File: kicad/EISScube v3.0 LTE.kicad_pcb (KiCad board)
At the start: 4 copper layers, 100 x 72 mm, 255 parts, among them J1 Boot, J2 UART, J3 JTag, J4 SIM_Card_w_det_sw, J5 USB_B_Mini, J6 Screw_Terminal_01x08, K1 SANYOU_SRD_Form_C, Q2 GSM3612PJZF, Q3 GSM3612PJZF, Q4 GSM3612PJZF, Q5 GSM3612PJZF, SW1 Reset, U1 STM32L051C8Tx, U2 SN74LV1T34DBVR, U3 U-Blox-SARA-R4, U4 LM2576HVS-12, U5 MIC29302WU-TR, U6 L7805, U7 LM1117-3.3, U8 LM1117-1.8, U9 LTV-357T, Y1 12MHz, Y2 32.768KHz

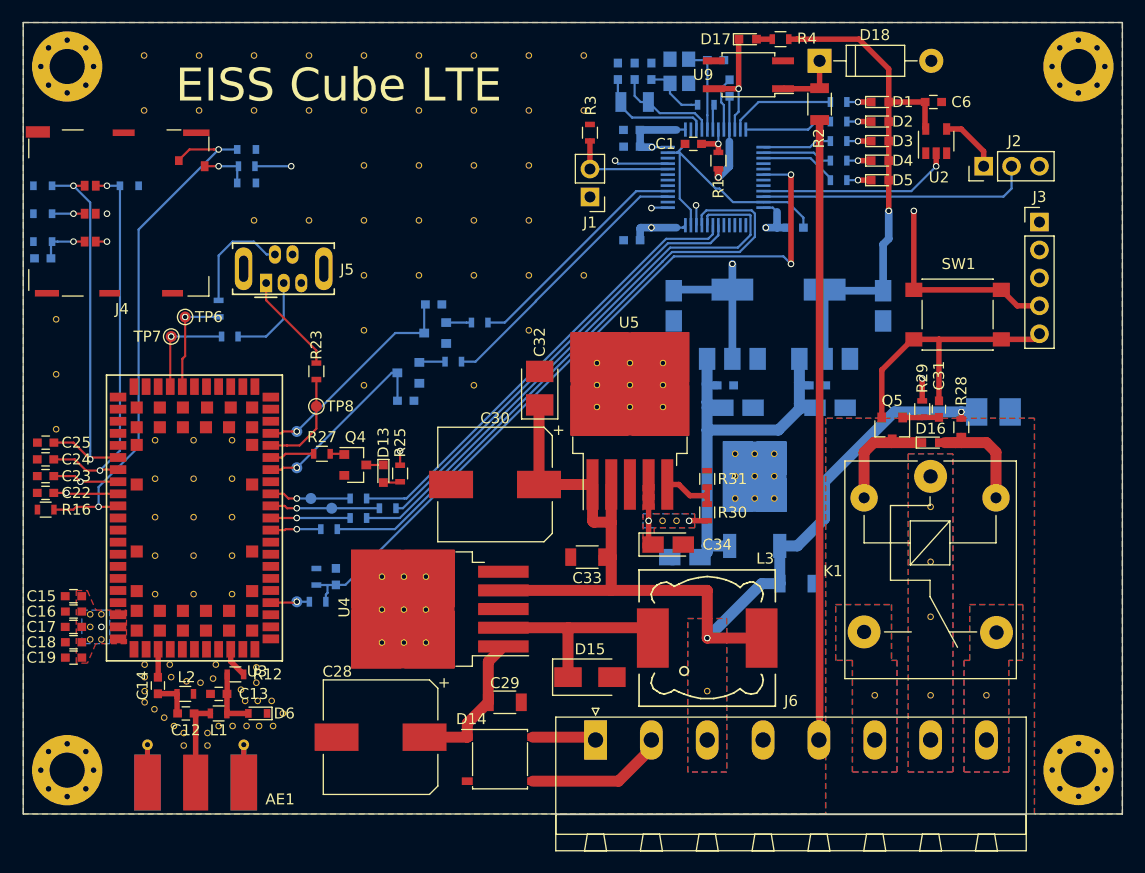
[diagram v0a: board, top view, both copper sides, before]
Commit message: Changes for enclosure case
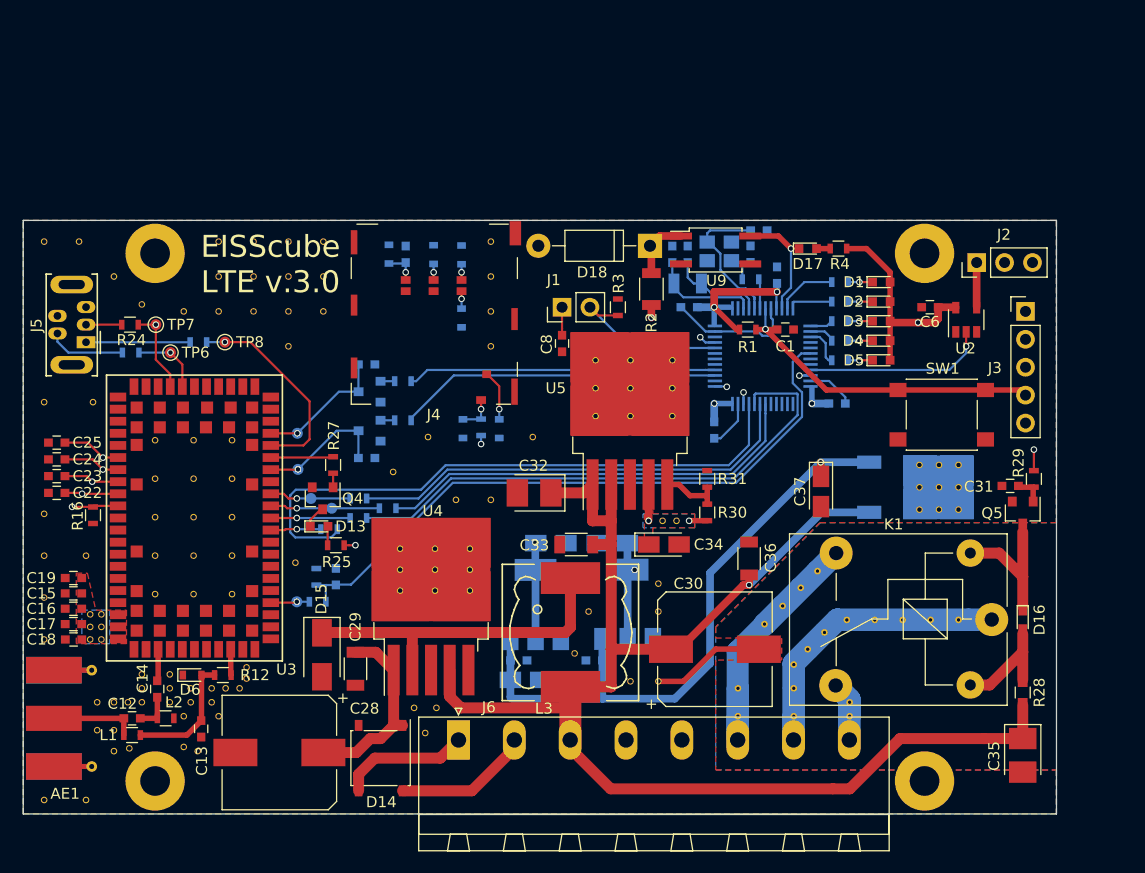
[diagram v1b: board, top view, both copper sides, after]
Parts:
- removed the REF** at (160.0, 122.2)
- removed the REF** at (180.3, 122.6)
- removed the REF** at (180.3, 115.4)
- removed the REF** at (180.3, 110.4)
- removed the REF** at (180.3, 105.4)
- removed the REF** at (185.4, 122.6)
- removed the REF** at (175.3, 122.6)
- removed the REF** at (128.8, 94.3)
- removed the REF** at (138.8, 94.3)
- removed the REF** at (143.8, 89.3)
- removed the REF** at (120.4, 123.1)
- removed the REF** at (121.4, 124.2)
- removed the REF** at (114.6, 126.0)
- removed the REF** at (115.1, 121.0)
- added REF**: VIA-0.6mm, EISScube_LTE:VIA-0.6mm, F.Cu at (134.4, 126.0)
- added REF**: VIA-0.6mm, EISScube_LTE:VIA-0.6mm, F.Cu at (104.9, 116.3)
- added REF**: VIA-0.6mm, EISScube_LTE:VIA-0.6mm, F.Cu at (170.1, 111.3)
- added REF**: VIA-0.6mm, EISScube_LTE:VIA-0.6mm, F.Cu at (168.5, 112.8)
- added REF**: VIA-0.6mm, EISScube_LTE:VIA-0.6mm, F.Cu at (166.9, 114.4)
- added REF**: VIA-0.6mm, EISScube_LTE:VIA-0.6mm, F.Cu at (165.2, 116.1)
- added REF**: VIA-0.6mm, EISScube_LTE:VIA-0.6mm, F.Cu at (173.0, 124.5)
- added REF**: VIA-0.6mm, EISScube_LTE:VIA-0.6mm, F.Cu at (173.0, 123.2)
- added REF**: VIA-0.6mm, EISScube_LTE:VIA-0.6mm, F.Cu at (162.8, 121.9)
- added REF**: VIA-0.6mm, EISScube_LTE:VIA-0.6mm, F.Cu at (162.8, 124.5)
- added REF**: VIA-0.6mm, EISScube_LTE:VIA-0.6mm, F.Cu at (169.2, 118.4)
- added REF**: VIA-0.6mm, EISScube_LTE:VIA-0.6mm, F.Cu at (167.9, 124.5)
- added REF**: VIA-0.6mm, EISScube_LTE:VIA-0.6mm, F.Cu at (175.3, 115.7)
- added REF**: VIA-0.6mm, EISScube_LTE:VIA-0.6mm, F.Cu at (135.4, 123.7)
- added REF**: VIA-0.6mm, EISScube_LTE:VIA-0.6mm, F.Cu at (177.8, 115.7)
- added REF**: VIA-0.6mm, EISScube_LTE:VIA-0.6mm, F.Cu at (167.9, 121.9)
- added REF**: VIA-0.6mm, EISScube_LTE:VIA-0.6mm, F.Cu at (167.9, 119.8)
- added REF**: VIA-0.6mm, EISScube_LTE:VIA-0.6mm, F.Cu at (170.7, 116.8)
- added REF**: VIA-0.6mm, EISScube_LTE:VIA-0.6mm, F.Cu at (172.7, 115.7)
- added REF**: VIA-0.6mm, EISScube_LTE:VIA-0.6mm, F.Cu at (180.3, 115.7)
- added REF**: VIA-0.6mm, EISScube_LTE:VIA-0.6mm, F.Cu at (182.9, 115.7)
- added REF**: VIA-0.6mm, EISScube_LTE:VIA-0.6mm, F.Cu at (133.3, 123.7)
- added REF**: VIA-0.6mm, EISScube_LTE:VIA-0.6mm, F.Cu at (148.0, 118.7)
- added REF**: VIA-0.6mm, EISScube_LTE:VIA-0.6mm, F.Cu at (149.2, 114.9)
- added REF**: VIA-0.6mm, EISScube_LTE:VIA-0.6mm, F.Cu at (155.6, 112.4)
- added REF**: VIA-0.6mm, EISScube_LTE:VIA-0.6mm, F.Cu at (155.6, 114.9)
- added REF**: VIA-0.6mm, EISScube_LTE:VIA-0.6mm, F.Cu at (155.6, 121.3)
- added REF**: VIA-0.6mm, EISScube_LTE:VIA-0.6mm, F.Cu at (153.0, 121.3)
- AE1: value Antenna_Shield -> Antenna
- C35, C36, C37, C8, R24: moved to F.Cu
- J4: value SIM_Card_w_det_sw -> SIM card holder
- J6: value Screw_Terminal_01x08 -> Connector 1 x 8
- K1: value SANYOU_SRD_Form_C -> SRD Form C
- R23: moved to B.Cu
- REF**: footprint Mounting_Holes:MountingHole_3.2mm_M3_Pad_Via -> Mounting_Holes:MountingHole_2.7mm_Pad
- REF** (x3): footprint Mounting_Holes:MountingHole_3.2mm_M3_Pad_Via -> Mounting_Holes:MountingHole_2.7mm_M2.5_Pad
- moved REF** 67.9 mm to (103.5, 132.1)
- moved REF** 63.4 mm to (99.7, 132.1)
- moved REF** 50.1 mm to (99.7, 117.5)
- moved REF** 49.2 mm to (99.7, 81.3)
- moved REF** 48.3 mm to (99.7, 113.7)
- moved REF** 48.0 mm to (103.5, 109.9)
- moved REF** 44.0 mm to (99.7, 106.0)
- moved D10 38.6 mm to (137.7, 82.5), turned to 270 degrees
- moved REF** 36.3 mm to (112.4, 87.6)
- moved D8 35.8 mm to (135.1, 82.5), turned to 270 degrees
- moved D11 34.3 mm to (141.1, 98.3), turned to 90 degrees
- moved REF** 33.9 mm to (108.6, 87.0)
- moved C41 33.2 mm to (149.1, 121.2), turned to 180 degrees
- moved REF** 33.1 mm to (122.6, 110.5)
- moved C21 33.0 mm to (132.6, 82.4), turned to 90 degrees
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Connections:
- D14 pad 3: 24VAC-2 -> 24VAC-1
- D14 pad 4: 24VAC-1 -> 24VAC-2
- J4 pad C6: Net-(J4-PadC6) -> (no net)
- J5 pad 4: Net-(J5-Pad4) -> (no net)
- U1 pad 16: Net-(U1-Pad16) -> (no net)
- U1 pad 17: Net-(U1-Pad17) -> (no net)
- U1 pad 19: Net-(U1-Pad19) -> (no net)
- U1 pad 2: Net-(U1-Pad2) -> (no net)
- U1 pad 20: Net-(U1-Pad20) -> (no net)
- U1 pad 25: Net-(U1-Pad25) -> (no net)
- U1 pad 26: Net-(U1-Pad26) -> (no net)
- U1 pad 27: Net-(U1-Pad27) -> (no net)
- U1 pad 28: Net-(U1-Pad28) -> (no net)
- U1 pad 29: Net-(U1-Pad29) -> (no net)
- U1 pad 38: Net-(U1-Pad38) -> (no net)
- U1 pad 41: Net-(U1-Pad41) -> (no net)
- U1 pad 42: Net-(U1-Pad42) -> (no net)
- U1 pad 43: Net-(U1-Pad43) -> (no net)
- U1 pad 46: Net-(U1-Pad46) -> (no net)
- U2 pad 1: Net-(U2-Pad1) -> (no net)
- U3 pad 19: Net-(U3-Pad19) -> (no net)
- U3 pad 2: Net-(U3-Pad2) -> (no net)
- U3 pad 23: Net-(U3-Pad23) -> (no net)
- U3 pad 24: Net-(U3-Pad24) -> (no net)
- U3 pad 25: Net-(U3-Pad25) -> (no net)
- U3 pad 26: Net-(U3-Pad26) -> (no net)
- U3 pad 27: Net-(U3-Pad27) -> (no net)
- U3 pad 31: Net-(U3-Pad31) -> (no net)
- U3 pad 33: Net-(U3-Pad33) -> (no net)
- U3 pad 34: Net-(U3-Pad34) -> (no net)
- U3 pad 35: Net-(U3-Pad35) -> (no net)
- U3 pad 36: Net-(U3-Pad36) -> (no net)
- U3 pad 37: Net-(U3-Pad37) -> (no net)
- U3 pad 44: Net-(U3-Pad44) -> (no net)
- U3 pad 45: Net-(U3-Pad45) -> (no net)
- U3 pad 46: Net-(U3-Pad46) -> (no net)
- U3 pad 47: Net-(U3-Pad47) -> (no net)
- U3 pad 48: Net-(U3-Pad48) -> (no net)
- U3 pad 49: Net-(U3-Pad49) -> (no net)
- U3 pad 6: Net-(U3-Pad6) -> (no net)
- U3 pad 7: Net-(U3-Pad7) -> (no net)
- U3 pad 8: Net-(U3-Pad8) -> (no net)
- U3 pad 9: Net-(U3-Pad9) -> (no net)
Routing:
- net /EISScube-pw/COM: track 0.00 -> 133.3 mm
- net /EISScube-pw/NC: track 0.07 -> 108.1 mm
- net +12V: track 93.1 -> 131.3 mm, vias 2 -> 1
- net /EISScube-pw/NO: track 0.00 -> 27.4 mm
- net GND: track 55.8 -> 30.8 mm, vias 1 -> 0
- net /EISScube-cl/V_INT: track 50.3 -> 27.0 mm
- net +1V8: track 100.9 -> 120.4 mm
- net /EISScube-pw/+5V: track 39.4 -> 58.5 mm, vias 0 -> 1
- net +3V3: track 48.0 -> 64.5 mm, vias 1 -> 2
- net /EISScube-cl/VSIM: track 33.6 -> 48.4 mm
- net INPUT: track 56.9 -> 43.1 mm, vias 0 -> 1
- net /EISScube-cl/SIM_RST: track 33.7 -> 47.3 mm
- net NRST: track 43.1 -> 30.0 mm, vias 2 -> 1
- net Net-(D15-Pad1): track 18.5 -> 30.8 mm
- net /EISScube-cl/SIM_CLK: track 35.0 -> 46.4 mm
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- removed copper zone on B.Cu, net +12V
- removed copper zone on F.Cu, net +12V
- removed copper zone on In1.Cu, net +12V
- removed copper zone on In2.Cu, net +12V
- removed copper zone on B.Cu, net /EISScube-pw/COM
- removed copper zone on F.Cu, net /EISScube-pw/COM
- removed copper zone on In1.Cu, net /EISScube-pw/COM
- removed copper zone on In2.Cu, net /EISScube-pw/COM
- removed copper zone on B.Cu, net /EISScube-pw/NC
- removed copper zone on F.Cu, net /EISScube-pw/NC
- removed copper zone on In1.Cu, net /EISScube-pw/NC
- removed copper zone on In2.Cu, net /EISScube-pw/NC
- removed copper zone on B.Cu, net /EISScube-pw/NO
- removed copper zone on F.Cu, net /EISScube-pw/NO
- removed copper zone on In1.Cu, net /EISScube-pw/NO
- removed copper zone on In2.Cu, net /EISScube-pw/NO
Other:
- board size 100 x 72 mm -> 94 x 54 mm
- board text added: "EISScube LTE v.3.0"
- board text removed: "EISS Cube LTE"
